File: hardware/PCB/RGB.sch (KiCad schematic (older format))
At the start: 28 parts, among them U1 IS31FL3733-QF, U2 IS31FL3733-QF

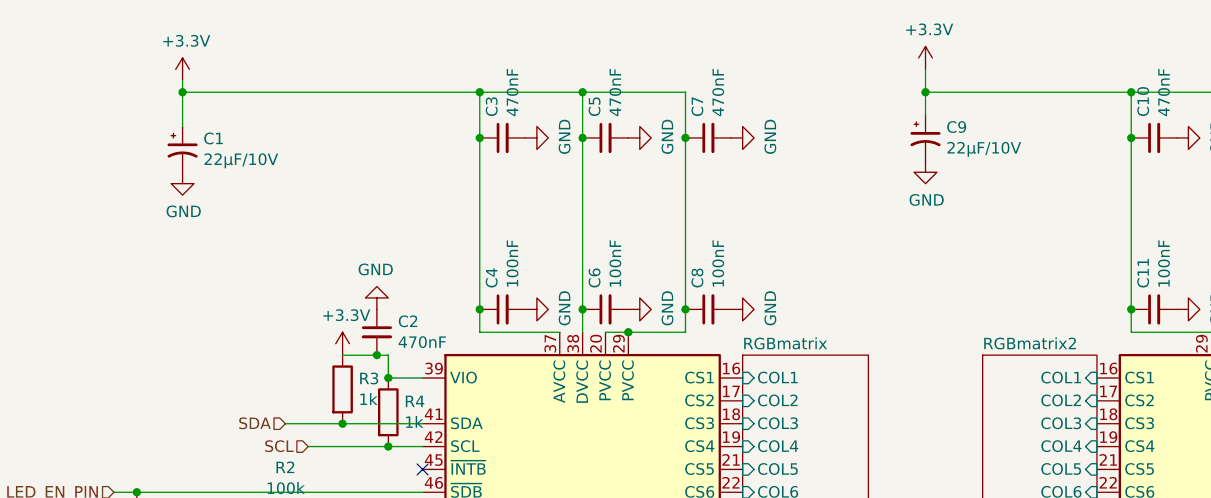
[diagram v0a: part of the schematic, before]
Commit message: getting closer to it actually works
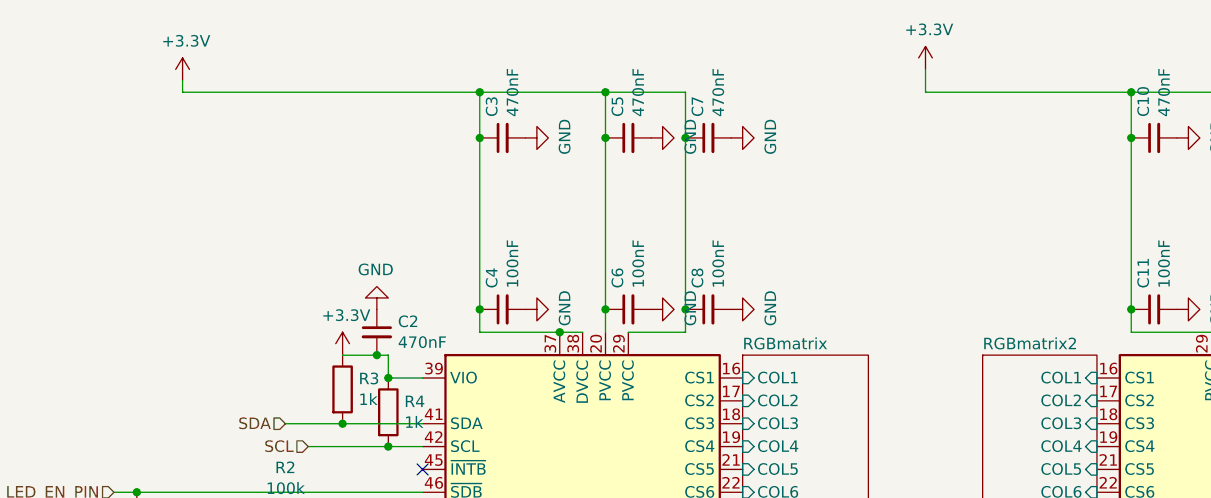
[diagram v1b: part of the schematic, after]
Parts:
- removed C1, C9: 22μF/10V, Capacitor_Tantalum_SMD:CP_EIA-3216-18_Kemet-A, symbol Device:CP1_Small
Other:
- moved on the sheet: C5, C6
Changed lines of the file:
@@
 Connection ~ 7000 950
 Connection ~ 6550 1150
-$Comp
-L Device:CP1_Small C9
-U 1 1 5E475E34
-P 5650 1150
-F 0 "C9" H 5741 1196 50  0000 L CNN
-F 1 "22μF/10V" H 5741 1105 50  0000 L CNN
-F 2 "Capacitor_Tantalum_SMD:CP_EIA-3216-18_Kemet-A" H 5650 1150 50  0001 C CNN
-F 3 "~" H 5650 1150 50  0001 C CNN
-F 4 "Capacitor_Tantalum_SMD:CP_EIA-3528-12_Kemet-T_Pad1.50x2.35mm_HandSolder" H 5650 1150 50  0001 C CNN "Footprint"
-F 5 "22μF/10V" H 5650 1150 50  0001 C CNN "Value"
-	1    5650 1150
-	1    0    0    -1
-$EndComp
-$Comp
-L power:GND #PWR016
-U 1 1 5E476AB6
-P 5650 1250
-F 0 "#PWR016" H 5650 1000 50  0001 C CNN
-F 1 "GND" H 5655 1077 50  0000 C CNN
-F 2 "" H 5650 1250 50  0001 C CNN
-F 3 "" H 5650 1250 50  0001 C CNN
-	1    5650 1250
-	1    0    0    -1
-$EndComp
 Connection ~ 6550 950
 $Comp
 L Device:C_Small C6
 U 1 1 5E48765C
-P 4250 1900
-F 0 "C6" H 4342 1946 50  0000 L CNN
-F 1 "100nF" H 4342 1855 50  0000 L CNN
-F 2 "Capacitor_SMD:C_0402_1005Metric" H 4250 1900 50  0001 C CNN
-F 3 "~" H 4250 1900 50  0001 C CNN
-F 4 "Capacitor_SMD:C_0603_1608Metric_Pad1.05x0.95mm_HandSolder" H 4250 1900 50  0001 C CNN "Footprint"
-F 5 "0.1μF" H 4250 1900 50  0001 C CNN "Value"
-	1    4250 1900
+P 4350 1900
+F 0 "C6" H 4442 1946 50  0000 L CNN
+F 1 "100nF" H 4442 1855 50  0000 L CNN
+F 2 "Capacitor_SMD:C_0402_1005Metric" H 4350 1900 50  0001 C CNN
+F 3 "~" H 4350 1900 50  0001 C CNN
+F 4 "Capacitor_SMD:C_0603_1608Metric_Pad1.05x0.95mm_HandSolder" H 4350 1900 50  0001 C CNN "Footprint"
+F 5 "0.1μF" H 4350 1900 50  0001 C CNN "Value"
+	1    4350 1900
 	0    -1   -1   0
 $EndComp
@@
 L power:GND #PWR012
 U 1 1 5E487662
-P 4350 1900
-F 0 "#PWR012" H 4350 1650 50  0001 C CNN
-F 1 "GND" H 4355 1727 50  0000 C CNN
-F 2 "" H 4350 1900 50  0001 C CNN
-F 3 "" H 4350 1900 50  0001 C CNN
-	1    4350 1900
+P 4450 1900
+F 0 "#PWR012" H 4450 1650 50  0001 C CNN
+F 1 "GND" H 4455 1727 50  0000 C CNN
+F 2 "" H 4450 1900 50  0001 C CNN
+F 3 "" H 4450 1900 50  0001 C CNN
+	1    4450 1900
 	0    -1   -1   0
 $EndComp
@@
 L Device:C_Small C5
 U 1 1 5E487668
-P 4250 1150
-F 0 "C5" H 4342 1196 50  0000 L CNN
-F 1 "470nF" H 4342 1105 50  0000 L CNN
-F 2 "Capacitor_SMD:C_0402_1005Metric" H 4250 1150 50  0001 C CNN
-F 3 "~" H 4250 1150 50  0001 C CNN
-F 4 "Capacitor_SMD:C_0603_1608Metric_Pad1.05x0.95mm_HandSolder" H 4250 1150 50  0001 C CNN "Footprint"
-F 5 "0.47μF" H 4250 1150 50  0001 C CNN "Value"
-	1    4250 1150
+P 4350 1150
+F 0 "C5" H 4442 1196 50  0000 L CNN
+F 1 "470nF" H 4442 1105 50  0000 L CNN
+F 2 "Capacitor_SMD:C_0402_1005Metric" H 4350 1150 50  0001 C CNN
+F 3 "~" H 4350 1150 50  0001 C CNN
+F 4 "Capacitor_SMD:C_0603_1608Metric_Pad1.05x0.95mm_HandSolder" H 4350 1150 50  0001 C CNN "Footprint"
+F 5 "0.47μF" H 4350 1150 50  0001 C CNN "Value"
+	1    4350 1150
 	0    -1   -1   0
 $EndComp
@@
 L power:GND #PWR011
 U 1 1 5E48766E
-P 4350 1150
-F 0 "#PWR011" H 4350 900 50  0001 C CNN
-F 1 "GND" H 4355 977 50  0000 C CNN
-F 2 "" H 4350 1150 50  0001 C CNN
-F 3 "" H 4350 1150 50  0001 C CNN
-	1    4350 1150
+P 4450 1150
+F 0 "#PWR011" H 4450 900 50  0001 C CNN
+F 1 "GND" H 4455 977 50  0000 C CNN
+F 2 "" H 4450 1150 50  0001 C CNN
+F 3 "" H 4450 1150 50  0001 C CNN
+	1    4450 1150
 	0    -1   -1   0
 $EndComp
@@
 $EndComp
 Wire Wire Line
-	4600 950  4150 950
-Wire Wire Line
-	4150 950  4150 1150
-Connection ~ 4150 1150
-Wire Wire Line
-	4150 950  3700 950
+	4600 950  4250 950
+Wire Wire Line
+	4250 950  4250 1150
+Connection ~ 4250 1150
 Wire Wire Line
 	3700 950  3700 1150
-Connection ~ 4150 950
 Connection ~ 3700 1150
 Wire Wire Line
@@
 Wire Wire Line
 	4600 2000 4350 2000
-Connection ~ 4350 2000
-Wire Wire Line
-	4350 2000 4250 2000
 Text HLabel 2100 2700 0    50   Input ~ 0
 LED_EN_PIN
@@
 Wire Wire Line
 	5650 850  5650 950
-Connection ~ 5650 950
-Wire Wire Line
-	5650 950  5650 1050
-$Comp
-L Device:CP1_Small C1
-U 1 1 5E6C50D8
-P 2400 1200
-F 0 "C1" H 2491 1246 50  0000 L CNN
-F 1 "22μF/10V" H 2491 1155 50  0000 L CNN
-F 2 "Capacitor_Tantalum_SMD:CP_EIA-3216-18_Kemet-A" H 2400 1200 50  0001 C CNN
-F 3 "~" H 2400 1200 50  0001 C CNN
-F 4 "Capacitor_Tantalum_SMD:CP_EIA-3528-12_Kemet-T_Pad1.50x2.35mm_HandSolder" H 2400 1200 50  0001 C CNN "Footprint"
-F 5 "22μF/10V" H 2400 1200 50  0001 C CNN "Value"
-	1    2400 1200
-	1    0    0    -1
-$EndComp
-$Comp
-L power:GND #PWR03
-U 1 1 5E6C50E2
-P 2400 1300
-F 0 "#PWR03" H 2400 1050 50  0001 C CNN
-F 1 "GND" H 2405 1127 50  0000 C CNN
-F 2 "" H 2400 1300 50  0001 C CNN
-F 3 "" H 2400 1300 50  0001 C CNN
-	1    2400 1300
-	1    0    0    -1
-$EndComp
 Wire Wire Line
 	2400 900  2400 950
-Connection ~ 2400 950
-Wire Wire Line
-	2400 950  2400 1100
 Connection ~ 3700 950
 Connection ~ 3700 1900
@@
 Wire Wire Line
 	3700 1150 3700 1900
-Connection ~ 4150 1900
-Wire Wire Line
-	4150 1900 4150 2000
-Wire Wire Line
-	4150 1150 4150 1900
+Connection ~ 4250 1900
+Wire Wire Line
+	4250 1900 4250 2000
+Wire Wire Line
+	4250 1150 4250 1900
 Connection ~ 4600 1900
 Wire Wire Line
@@
 NoConn ~ 6400 3600
 NoConn ~ 4850 3600
+Wire Wire Line
+	4150 2000 4050 2000
+Connection ~ 4050 2000
+Connection ~ 4250 950
+Wire Wire Line
+	3700 950  4250 950
 $EndSCHEMATC
